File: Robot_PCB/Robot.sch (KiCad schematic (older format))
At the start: 2 parts

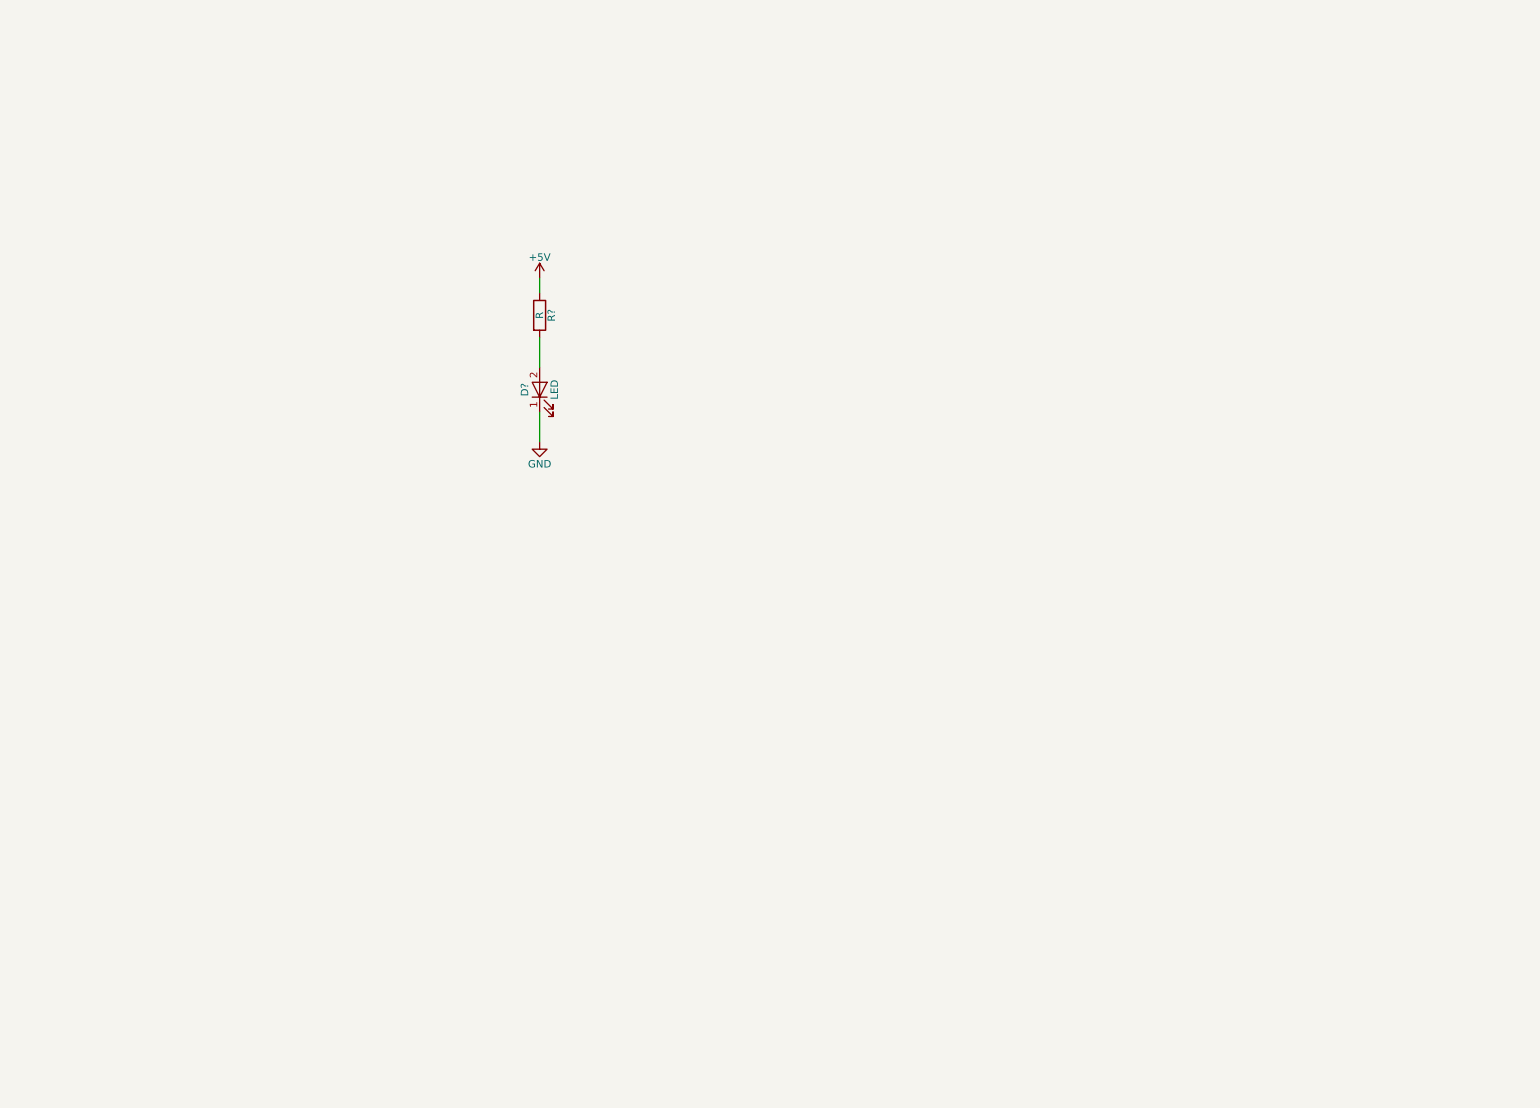
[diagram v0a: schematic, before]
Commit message: Robot
Shema robota kiCAD in pdf
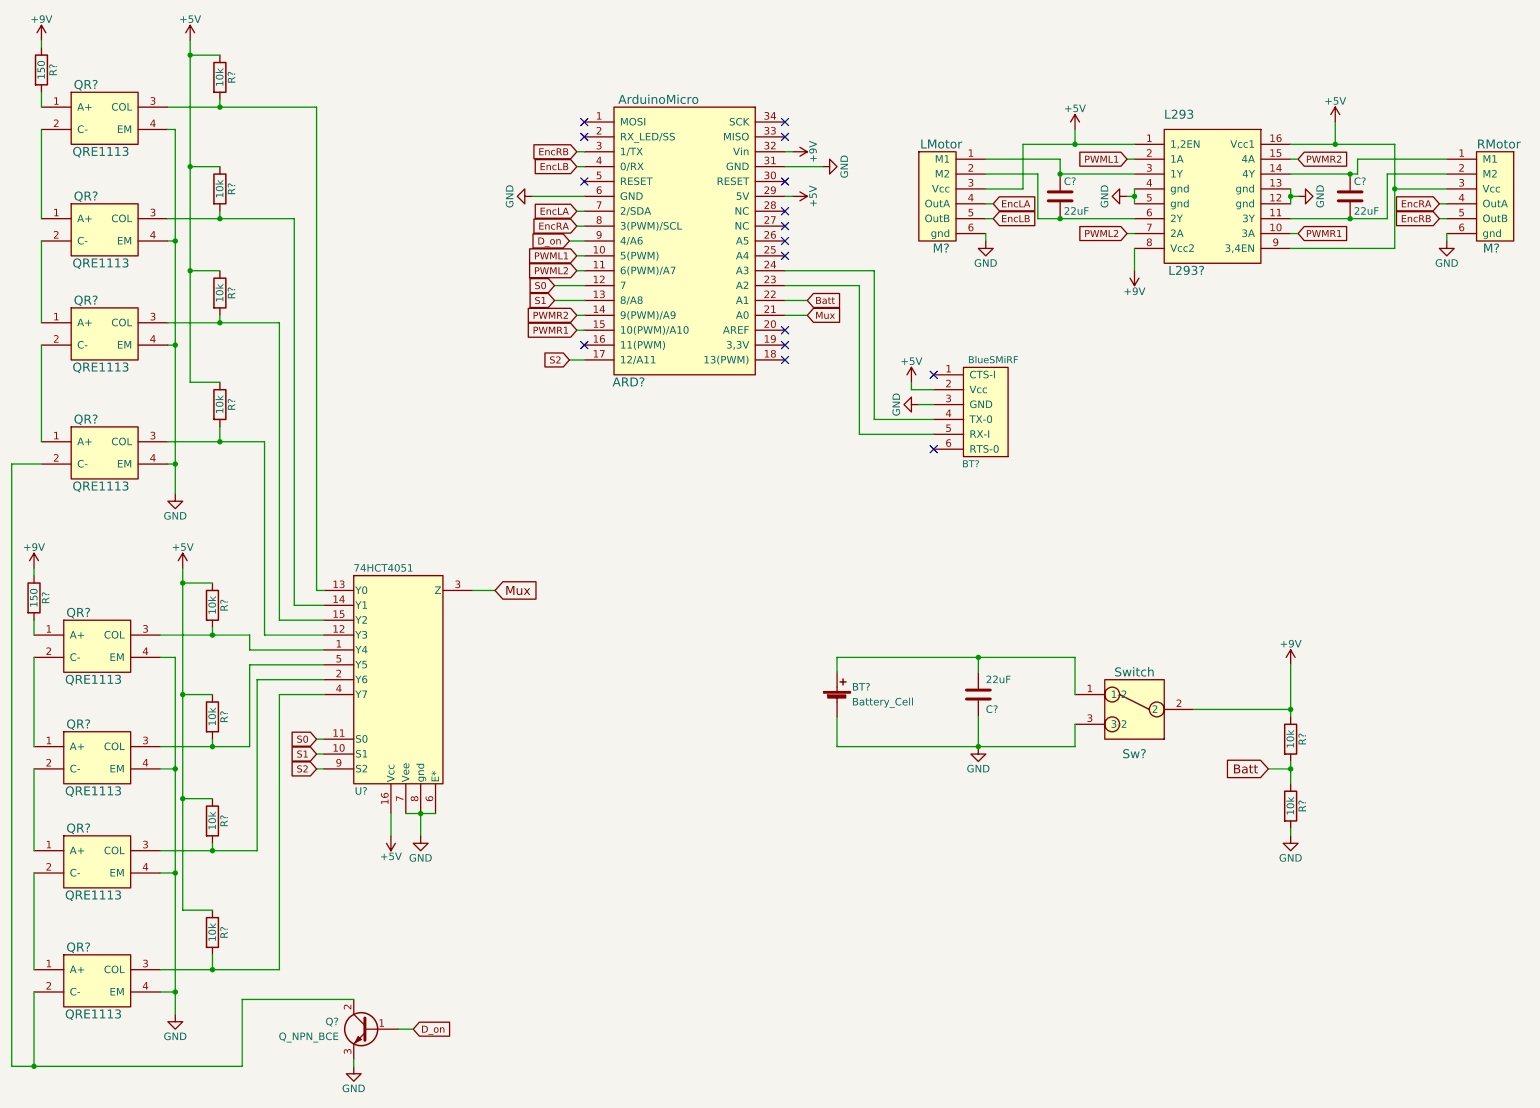
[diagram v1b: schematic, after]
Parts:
- removed D?: LED, symbol LED
- removed R?: R, symbol R
- added ARD?: ArduinoMicro, symbol ArduinoMicro
- added BT?: BlueSMiRF, symbol BlueSMiRF
- added BT?: Battery_Cell, symbol Battery_Cell
- added C? (x3): 22uF, symbol C
- added L293?: L293, symbol L293
- added M?: RMotor, symbol Motor
- added M?: LMotor, symbol Motor
- added Q?: Q_NPN_BCE, symbol Q_NPN_BCE
- added QR? (x8): QRE1113, symbol QRE1113
- added R? (x2): 150, symbol R
- added R? (x10): 10k, symbol R
- added Sw?: Switch, symbol Switch
- added U?: 74HCT4051, symbol 74HCT4051
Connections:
- net +5V: now also ARD?.29 (5V), BT?.2 (Vcc), L293?.1 (1,2EN), L293?.16 (Vcc1), L293?.9 (3,4EN), M?.3 (Vcc), M?.3 (Vcc), R?.1, R?.1, R?.1, R?.1, R?.1, R?.1, R?.1, R?.1, U?.16 (Vcc)
- net GND: now also ARD?.31 (GND), ARD?.6 (GND), BT?.2 (-), BT?.3 (GND), C?.2, L293?.12 (gnd), L293?.13 (gnd), L293?.4 (gnd), L293?.5 (gnd), M?.6 (gnd), M?.6 (gnd), Q?.3 (E), QR?.4 (EM), QR?.4 (EM), QR?.4 (EM), QR?.4 (EM), QR?.4 (EM), QR?.4 (EM), QR?.4 (EM), QR?.4 (EM), R?.2, Sw?.3 (3-2), U?.6 (E*), U?.7 (Vee), U?.8 (gnd)
- new net: QR?.1 (A+), QR?.2 (C-) (x6)
- new net: QR?.3 (COL), R?.2, U?.5 (Y5)
- new net: QR?.3 (COL), R?.2, U?.2 (Y6)
- new net: Q?.2 (C), QR?.2 (C-), QR?.2 (C-)
- new net: QR?.3 (COL), R?.2, U?.4 (Y7)
- new net: QR?.1 (A+), R?.2 (x2)
- new net: QR?.3 (COL), R?.2, U?.1 (Y4)
- new net: QR?.3 (COL), R?.2, U?.14 (Y1)
- new net: QR?.3 (COL), R?.2, U?.15 (Y2)
- new net: QR?.3 (COL), R?.2, U?.12 (Y3)
- new net: QR?.3 (COL), R?.2, U?.13 (Y0)
- new net: ARD?.23 (A2), BT?.5 (RX-I)
- new net: ARD?.24 (A3), BT?.4 (TX-0)
- new net: C?.2, L293?.11 (3Y), M?.2 (M2)
- new net: C?.1, L293?.14 (4Y), M?.1 (M1)
- new net: C?.1, L293?.3 (1Y), M?.1 (M1)
- new net: C?.2, L293?.6 (2Y), M?.2 (M2)
- new net: BT?.1 (+), C?.1, Sw?.1 (1-2)
- new net +9V: ARD?.32 (Vin), L293?.8 (Vcc2), R?.1, R?.1, R?.1, Sw?.2
- new net Batt: ARD?.22 (A1), R?.1, R?.2
- new net D_on: ARD?.9 (4/A6), Q?.1 (B)
- new net EncLA: ARD?.7 (2/SDA), M?.4 (OutA)
- new net EncLB: ARD?.4 (0/RX), M?.5 (OutB)
- new net EncRA: ARD?.8 (3(PWM)/SCL), M?.4 (OutA)
- new net EncRB: ARD?.3 (1/TX), M?.5 (OutB)
- new net Mux: ARD?.21 (A0), U?.3 (Z)
- new net PWML1: ARD?.10 (5(PWM)), L293?.2 (1A)
- new net PWML2: ARD?.11 (6(PWM)/A7), L293?.7 (2A)
- new net PWMR1: ARD?.15 (10(PWM)/A10), L293?.10 (3A)
- new net PWMR2: ARD?.14 (9(PWM)/A9), L293?.15 (4A)
- new net S0: ARD?.12 (7), U?.11 (S0)
- new net S1: ARD?.13 (8/A8), U?.10 (S1)
- new net S2: ARD?.17 (12/A11), U?.9 (S2)
- no-connect marks 0 -> 16
